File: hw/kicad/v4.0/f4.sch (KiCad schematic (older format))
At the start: 33 parts, among them P1 USB_OTG, U1 USBLC6-4SC6, U26 STM32F405VG, Y2 8M

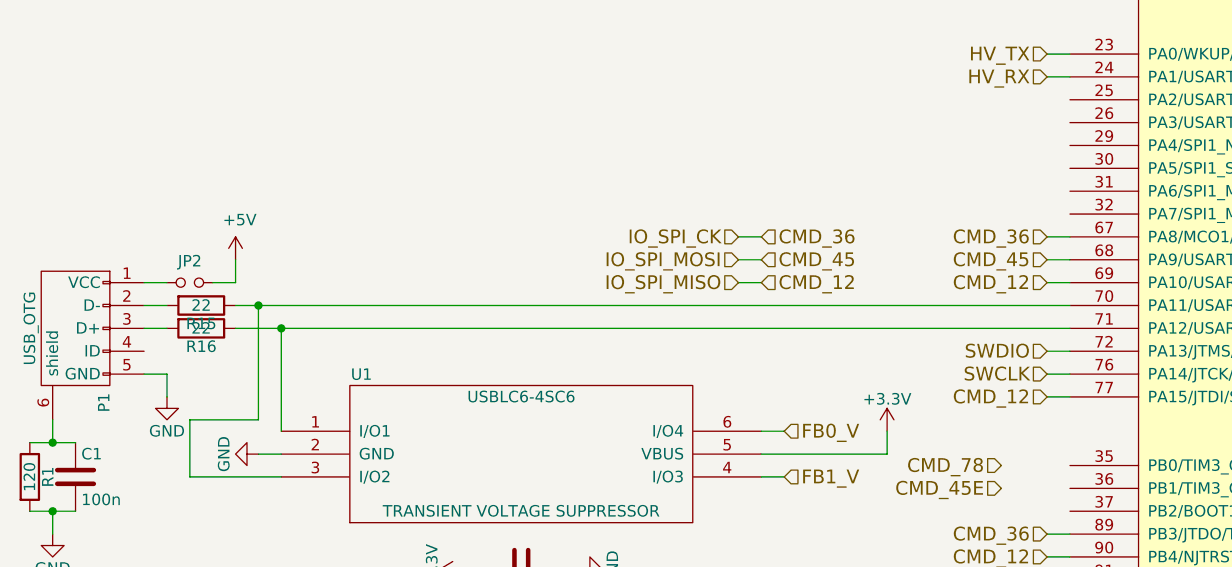
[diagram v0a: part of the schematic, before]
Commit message: v4.0
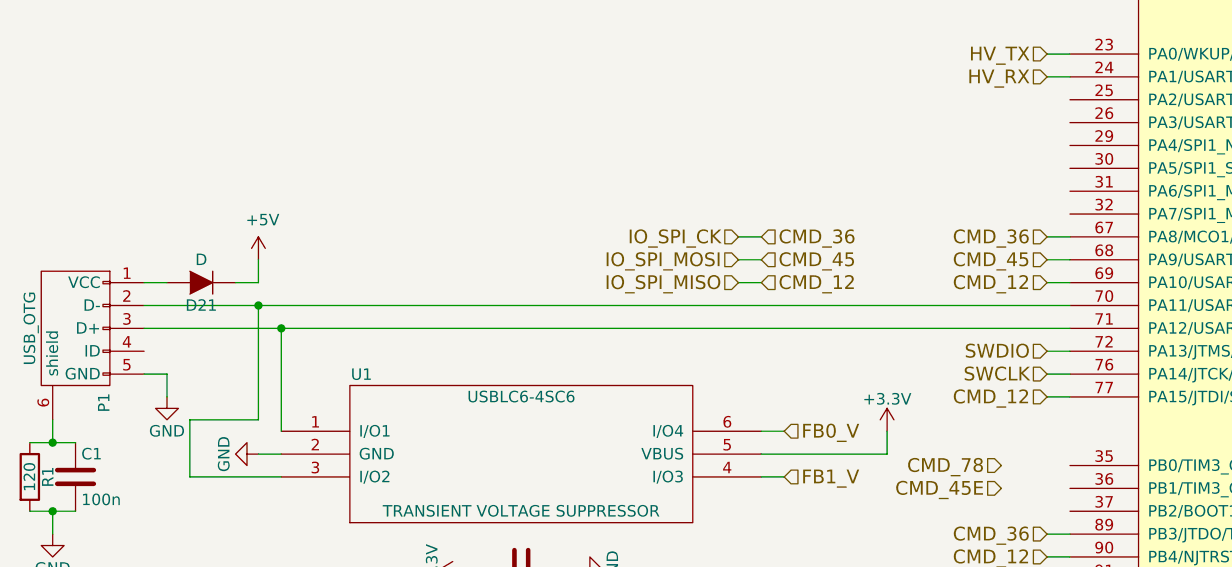
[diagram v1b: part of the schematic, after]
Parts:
- removed JP2: Jumper_NO_Small, symbol Jumper_NO_Small
- removed R15, R16: 22, stmbl:R_0603, symbol R
- added D21: D, Diodes_SMD:SMA_Standard, symbol D
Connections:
- net +5V: now also D21.1 (K)
- net at U1.3 (I/O2), U26.70 (PA11/USART1_CTS/CAN1_RX/TIM1_CH4_/OTG_FS_DM/EVENTOUT): now also P1.2 (D-)
- net at U1.1 (I/O1), U26.71 (PA12/USART1_RTS/CAN1_TX/TIM1_ETR/OTG_FS_DP/EVENTOUT): now also P1.3 (D+)
- net at P1.1 (VCC): now also D21.2 (A)
